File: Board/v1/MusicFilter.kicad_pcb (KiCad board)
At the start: 4 copper layers, 60 x 60 mm, 51 parts, among them J1 TYPE-C-31-M-17, J2 FPC 0.5mm 10P, J3 Conn_01x08_Male, J4 Conn_01x02_Male, P1 SWDPins, SW1 SW_Push, SW2 SW_Push, U1 MP2359, U2 STM32F103CBUx, Y1 8MHz

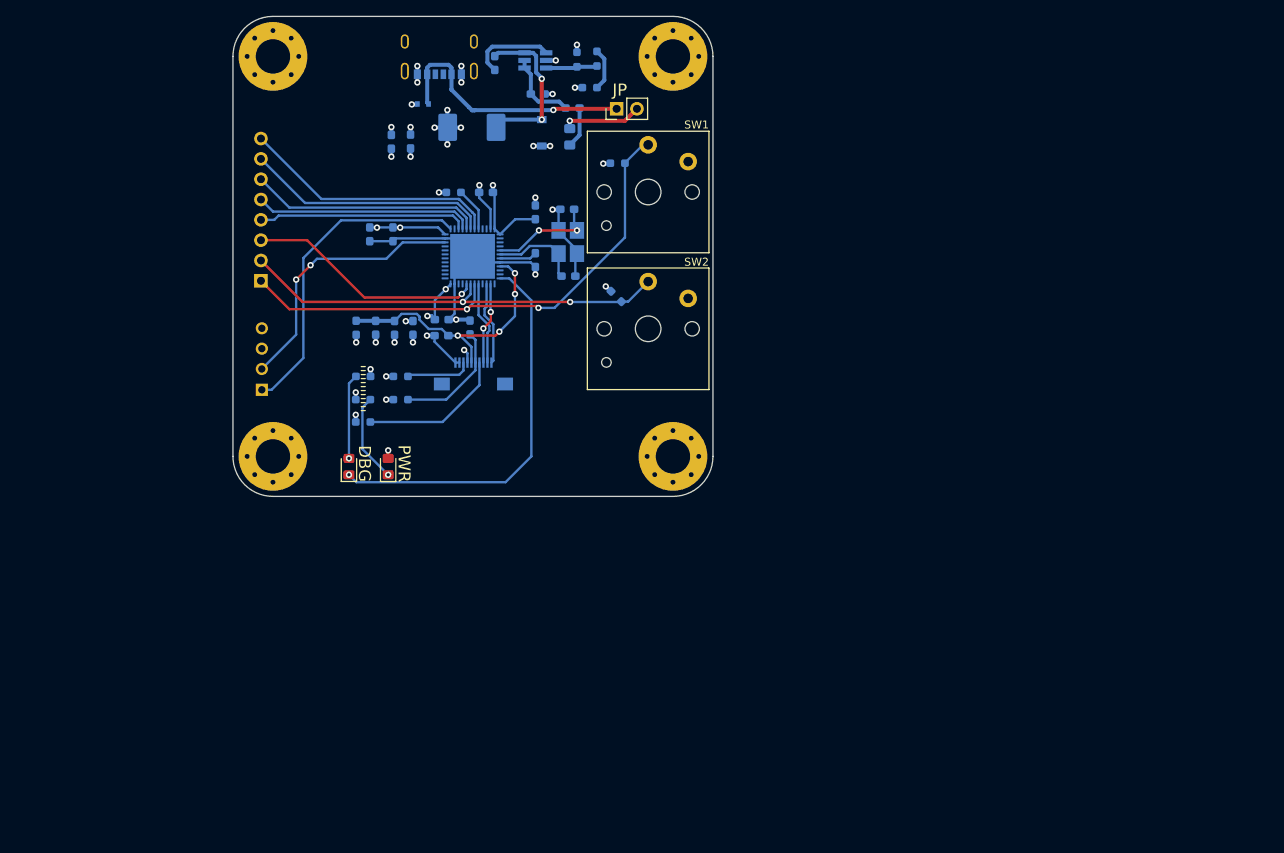
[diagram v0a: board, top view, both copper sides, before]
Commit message: board v2 is out
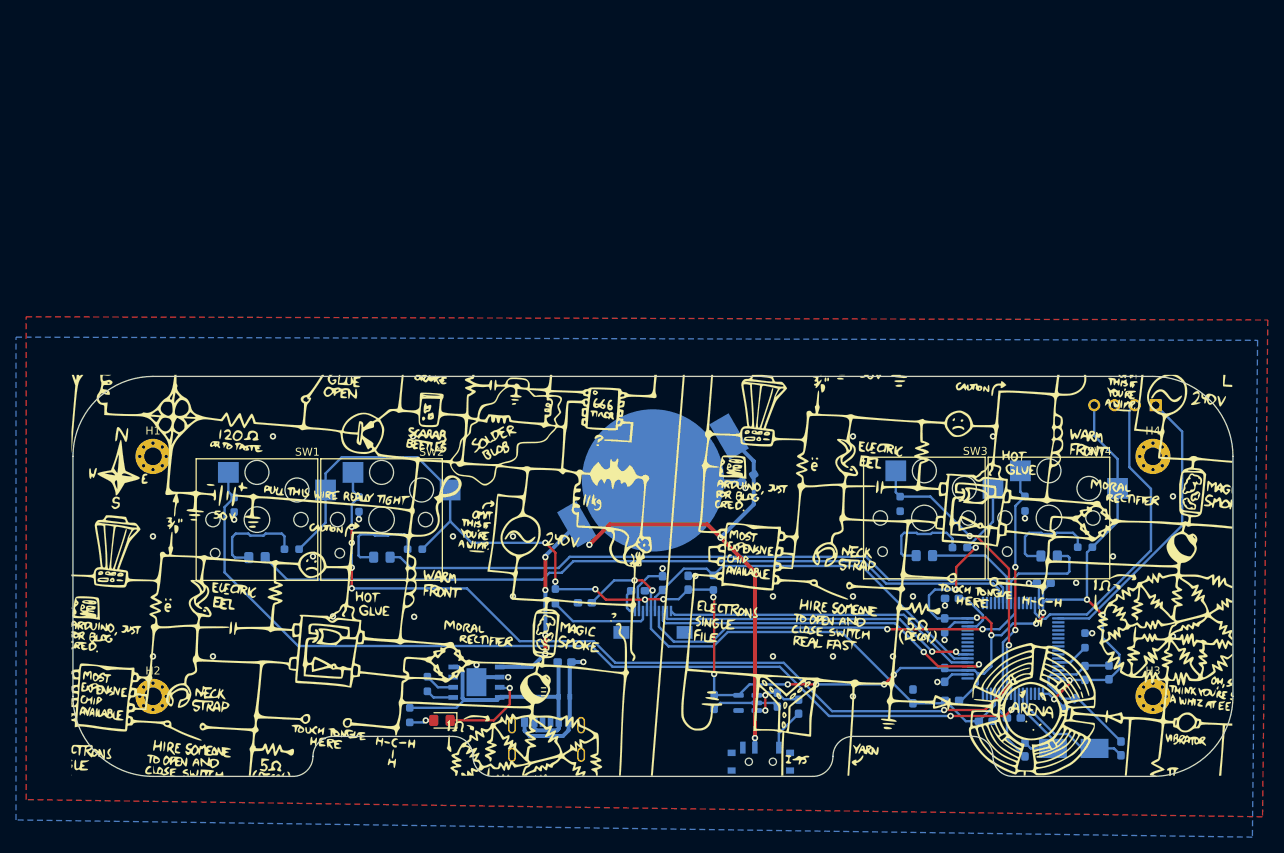
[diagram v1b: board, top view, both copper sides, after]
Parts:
- removed DECO**: Val**, DannyFootprintLibs:FOR_TEST
- removed FB2: 600 @ 100 MHz, Inductor_SMD:L_0603_1608Metric_Pad1.05x0.95mm_HandSolder
- removed J3: Conn_01x08_Male, Connector_PinHeader_2.54mm:PinHeader_1x08_P2.54mm_Vertical
- removed J4: Conn_01x02_Male, Connector_PinHeader_2.54mm:PinHeader_1x02_P2.54mm_Vertical
- removed L1: 47u, Inductor_SMD:L_Abracon_ASPI-0630LR
- added BT1: BK-912, DannyFootprintLibs:BK-912, B.Cu at (97.5, 103.0)
- added C18: 1u, Capacitor_SMD:C_0603_1608Metric_Pad1.08x0.95mm_HandSolder, B.Cu at (101.9, 115.8)
- added C19: 100n, Capacitor_SMD:C_0603_1608Metric_Pad1.08x0.95mm_HandSolder, B.Cu at (98.7, 115.8)
- added C20: 100n, Capacitor_SMD:C_0603_1608Metric_Pad1.08x0.95mm_HandSolder, B.Cu at (95.6, 116.8)
- added D5: WHITE, LED_SMD:LED_0805_2012Metric_Pad1.15x1.40mm_HandSolder, B.Cu at (131.4, 112.4)
- added D6: WHITE, LED_SMD:LED_0805_2012Metric_Pad1.15x1.40mm_HandSolder, B.Cu at (147.0, 112.5)
- added IC1: TP4056X, DannyFootprintLibs:ESOP-8_L4.9-W3.9-P1.27-LS6.0-BL-EP, B.Cu at (75.4, 128.2)
- added R12: 1k5, Resistor_SMD:R_0603_1608Metric_Pad0.98x0.95mm_HandSolder, B.Cu at (135.8, 111.4)
- added R13: 1k5, Resistor_SMD:R_0603_1608Metric_Pad0.98x0.95mm_HandSolder, B.Cu at (151.5, 111.3)
- added Ref**: Val**, DannyFootprintLibs:PIC_Sche2, F.Cu at (97.3, 114.8)
- added SW3: SW_Push, DannyFootprintLibs:SW_Kailh_Choc_V1_HOTSWAP, F.Cu at (131.4, 107.7)
- added SW4: SW_Push, DannyFootprintLibs:SW_Kailh_Choc_V1_HOTSWAP, F.Cu at (147.0, 107.7)
- added SW5: SW_SPDT, Button_Switch_SMD:SW_SPDT_PCM12, B.Cu at (111.0, 137.8)
- C1: value 10n -> 22p
- C10, C13, C14: value 1u -> 100n
- C11: value 10n -> 100n
- C15, C16: value 12p -> 1u
- C17: value 100n -> 1u
- C4: value 10u -> 1u
- C5: value 4u7 -> 100n
- C6, C9: value 100n -> 4u7
- C7: value 100n -> 22p
- D1: value B5819W -> WHITE; footprint Diode_SMD:D_SOD-123 -> LED_SMD:LED_0805_2012Metric_Pad1.15x1.40mm_HandSolder; moved to F.Cu
- D3: value RED -> WHITE; moved to B.Cu
- D4: value BLUE -> WHITE; moved to B.Cu
- F1: value 500mA -> 200mA; footprint Fuse:Fuse_0805_2012Metric_Pad1.15x1.40mm_HandSolder -> Fuse:Fuse_0603_1608Metric_Pad1.05x0.95mm_HandSolder
- H1, H2, H3, H4: value MountingHole_Pad -> MH; footprint MountingHole:MountingHole_4.3mm_M4_Pad_Via -> MountingHole:MountingHole_2.2mm_M2_Pad_Via
- J1: value TYPE-C-31-M-17 -> FPC 0.5mm 10P; footprint DannyFootprintLibs:TYPE-C-SMD_TYPE-C-31-M-16 -> DannyFootprintLibs:96x96 Sharp Memory Lcd With FPC Connector 10p 0.5mm; moved to F.Cu
- J2: value FPC 0.5mm 10P -> TYPE-C-31-M-17; footprint DannyFootprintLibs:FPC 0.5mm 10P -> DannyFootprintLibs:TYPE-C-SMD_TYPE-C-31-M-16
- R10, R11: value 10k -> 1k5
- R2: value 15k -> 1k5
- R3: value 270 -> 17k4
- R5: value 1k5 -> 10k
- R9: value 1k -> 10k
- SW1, SW2: footprint DannyFootprintLibs:SW_Kailh_Choc_V1 -> DannyFootprintLibs:SW_Kailh_Choc_V1_HOTSWAP
- U1: value MP2359 -> STM32F401RCTx; footprint Package_TO_SOT_SMD:SOT-23-6_Handsoldering -> Package_QFP:LQFP-64_10x10mm_P0.5mm
- U2: value STM32F103CBUx -> LP5907MFX-3.3; footprint Package_DFN_QFN:QFN-48-1EP_7x7mm_P0.5mm_EP5.6x5.6mm -> Package_TO_SOT_SMD:SOT-23-5
- Y1: value 8MHz -> 8MHz 20pF; footprint Crystal:Crystal_SMD_3225-4Pin_3.2x2.5mm_HandSoldering -> Crystal:Crystal_SMD_5032-2Pin_5.0x3.2mm_HandSoldering
- moved C1 116.0 mm to (156.0, 136.5), turned to 90 degrees
- moved H3 114.0 mm to (160.0, 130.0)
- moved P1 104.5 mm to (152.7, 93.6), turned to -90 degrees
- moved H2 103.1 mm to (35.0, 130.0)
- moved C7 101.9 mm to (144.0, 136.6)
- moved C5 100.7 mm to (142.6, 132.7), turned to 180 degrees
- moved C13 96.5 mm to (151.5, 127.1), turned to 90 degrees
- moved R1 96.5 mm to (151.5, 123.0)
- moved C4 95.2 mm to (130.0, 130.0)
- moved U1 94.7 mm to (142.5, 124.0), turned to 90 degrees
- moved C9 91.9 mm to (154.5, 127.0)
- moved C11 91.0 mm to (149.6, 130.9), turned to 45 degrees
- moved C8 90.9 mm to (139.1, 133.1), turned to 0 degrees
- moved Y1 89.5 mm to (150.1, 136.5), turned to 180 degrees
- moved C10 89.4 mm to (146.3, 115.8), turned to 180 degrees
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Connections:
- C1 pad 1: BUCK_SW -> OSC_IN
- C1 pad 2: BUCK_BST -> GND
- C10 pad 1: +3.3VA -> +3V3
- C11 pad 1: +3.3VA -> +3V3
- C12 pad 1: DISP -> +3V3
- C13 pad 1: +3.3VA -> +3V3
- C15 pad 1: OSC_IN -> Net-(C15-Pad1)
- C16 pad 1: OSC_OUT -> +3V3
- C17 pad 1: NRST -> +3.3VA
- C2 pad 1: BUCK_EN -> 5V
- C3 pad 2: +3V3 -> BAT
- C4 pad 1: GND -> +3.3VA
- C4 pad 2: +3V3 -> GND
- C5 pad 1: +3V3 -> NRST
- C6 pad 1: +3V3 -> VCAP1
- C7 pad 1: +3V3 -> OSC_OUT
- C8 pad 1: +3V3 -> +3.3VA
- D1 pad 1: BUCK_SW -> CHRG
- D1 pad 2: GND -> Net-(D1-Pad2)
- D2 pad 1: +5V -> 5V
- D3 pad 1: Net-(D3-Pad1) -> KEY1_LED
- D3 pad 2: +3V3 -> Net-(D3-Pad2)
- D4 pad 1: LED_STATUS -> KEY2_LED
- F1 pad 1: Net-(F1-Pad1) -> LDO_IN
- F1 pad 2: Net-(F1-Pad2) -> Net-(C15-Pad1)
- FB1 pad 1: Net-(F1-Pad2) -> +3V3
- FB1 pad 2: BUCK_EN -> +3.3VA
- J1 pad 1: unconnected-(J1-Pad1) -> SPI1_CLK
- J1 pad 2: unconnected-(J1-Pad2) -> SPI1_MOSI
- J1 pad 3: unconnected-(J1-Pad3) -> CS
- J1 pad 4: unconnected-(J1-Pad4) -> EXTCOMM
- J2 pad 1: SPI1_CLK -> unconnected-(J2-Pad1)
- J2 pad 2: SPI1_MOSI -> unconnected-(J2-Pad2)
- J2 pad 3: CS -> unconnected-(J2-Pad3)
- J2 pad 4: EXTCOMM -> unconnected-(J2-Pad4)
- R1 pad 1: BUCK_FB -> BOOT0
- R1 pad 2: +3V3 -> GND
- R10 pad 1: /KEY1 -> Net-(D3-Pad2)
- R10 pad 2: GND -> +3V3
- R11 pad 1: GND -> Net-(D4-Pad2)
- R11 pad 2: /KEY2 -> +3V3
- R2 pad 1: Net-(R2-Pad1) -> Net-(D1-Pad2)
- R2 pad 2: BUCK_FB -> 5V
- R3 pad 2: Net-(R2-Pad1) -> PROG
- R4 pad 1: DISP -> KEY1
- R4 pad 2: +3V3 -> GND
- R5 pad 2: Net-(D3-Pad1) -> KEY2
- R6 pad 1: EXTCOMM -> KEY3
- R7 pad 1: EXTMODE -> GND
- R7 pad 2: GND -> KEY4
- R8 pad 1: BOOT0 -> DISP
- R8 pad 2: GND -> +3V3
- R9 pad 1: Net-(D4-Pad2) -> EXTMODE
- SW1 pad 1: /KEY1 -> KEY1
- SW2 pad 1: /KEY2 -> KEY2
- U1 pad 1: BUCK_BST -> +3V3
- U1 pad 2: GND -> unconnected-(U1-Pad2)
- U1 pad 3: BUCK_FB -> unconnected-(U1-Pad3)
- U1 pad 4: BUCK_EN -> unconnected-(U1-Pad4)
- U1 pad 5: BUCK_EN -> OSC_IN
- U1 pad 6: BUCK_SW -> OSC_OUT
- U2 pad 1: +3V3 -> Net-(C15-Pad1)
- U2 pad 2: unconnected-(U2-Pad2) -> GND
- U2 pad 3: unconnected-(U2-Pad3) -> Net-(C15-Pad1)
- U2 pad 5: OSC_IN -> +3V3
- Y1 pad 2: GND -> OSC_OUT
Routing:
- net +3V3: track 44.8 -> 239.5 mm, vias 18 -> 21
- net KEY1: track 0.00 -> 121.6 mm, vias 0 -> 2
- net KEY2: track 0.00 -> 107.4 mm, vias 0 -> 6
- net KEY1_LED: track 0.00 -> 97.0 mm
- net BAT: track 0.00 -> 89.2 mm, vias 0 -> 7
- net KEY2_LED: track 0.00 -> 81.3 mm
- net /KEY1: track 67.6 -> 0.00 mm, vias 2 -> 0
- net /KEY2: track 54.3 -> 0.00 mm, vias 2 -> 0
- net LED_STATUS: track 49.1 -> 0.00 mm, vias 1 -> 0
- net 5V: track 0.00 -> 36.7 mm
- net KEY3: track 0.00 -> 36.5 mm, vias 0 -> 2
- net CS: track 10.2 -> 44.7 mm
- net DISP: track 14.7 -> 47.9 mm
- net +3.3VA: track 34.4 -> 66.9 mm, vias 4 -> 2
- net +5V: track 32.5 -> 0.00 mm, vias 1 -> 0
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- added copper zone on B.Cu, net GND
- added copper zone on F.Cu, net GND
- removed copper zone on In2.Cu, net +3V3
- removed copper zone on In1.Cu, net GND
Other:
- board size 60 x 60 mm -> 145 x 50 mm
- copper layers 4 -> 2
- board text removed: "DBG"
- board text removed: "JP"
- board text removed: "PWR"
